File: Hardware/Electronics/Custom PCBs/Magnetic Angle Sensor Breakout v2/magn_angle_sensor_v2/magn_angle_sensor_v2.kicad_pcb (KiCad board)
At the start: 2 copper layers, 25 x 25 mm, 57 parts, among them J1 JST PH 01x04, J2 USB C Receptacle, J3 120TR, SW1 USB_BOOT, SW2 RESET, U1 MT6701-CT, U2 RP2040, U3 W25Q128JVS, U4 SE8650X2-HF, U5 SN65HVD1050D, U6 XC6206P332MR, Y1 12MHz/12pF/50Ω/20ppm

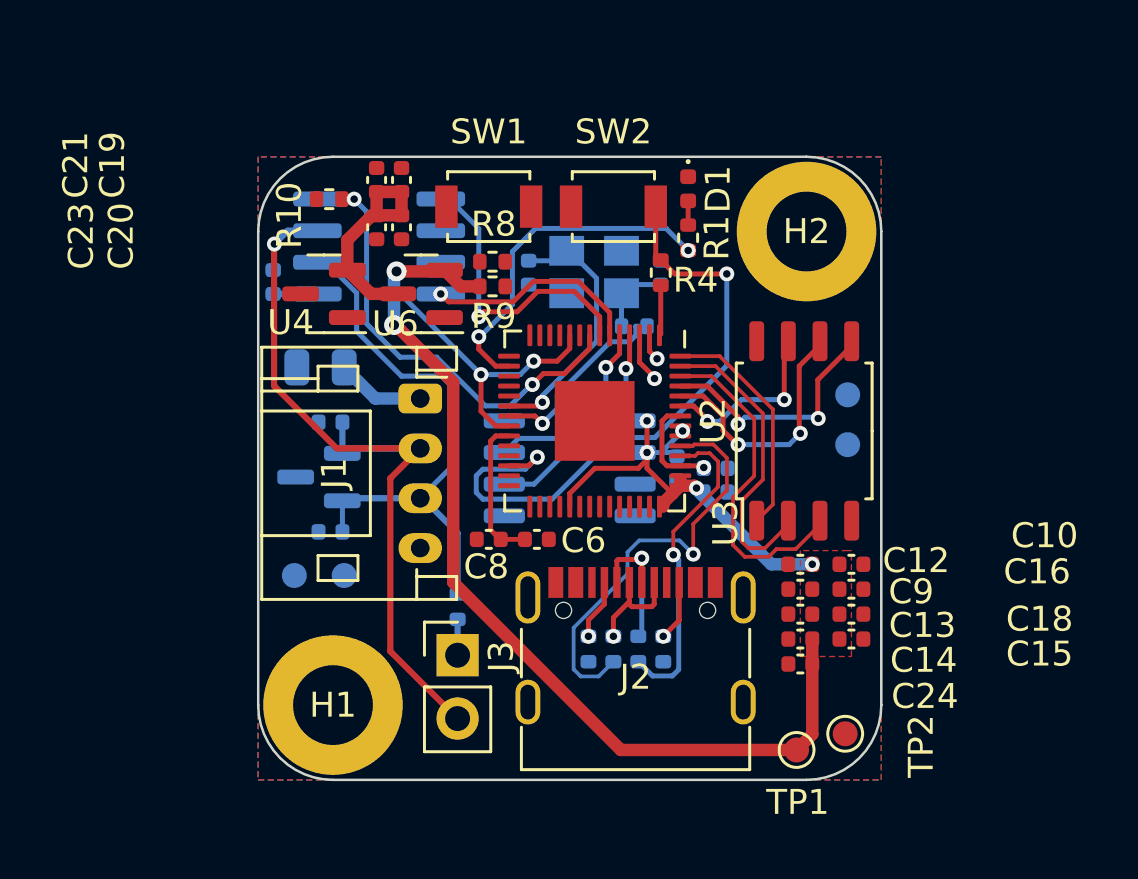
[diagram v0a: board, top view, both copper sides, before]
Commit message: Finish CAN Magnetic Angle Sensor v2
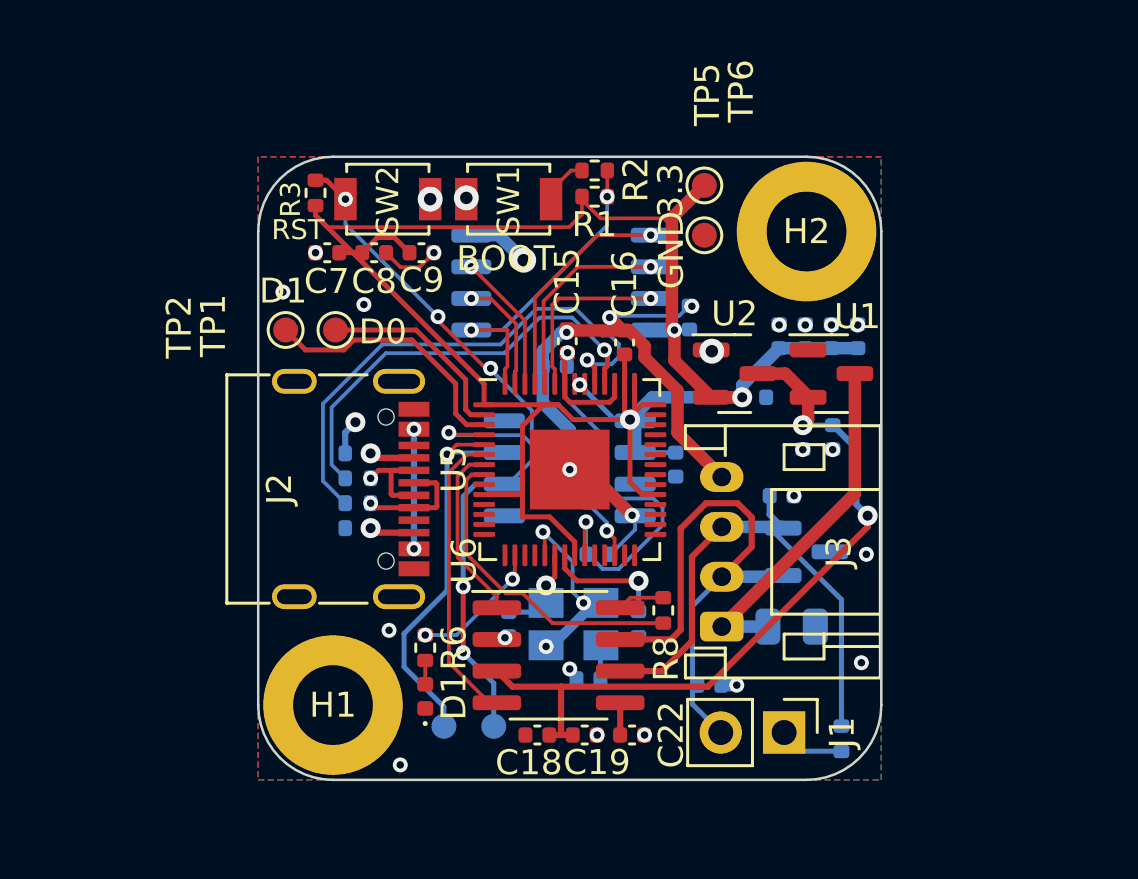
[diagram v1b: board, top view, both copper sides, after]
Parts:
- C10: value 100n -> 1u/100V; footprint Capacitor_SMD:C_0402_1005Metric -> Capacitor_SMD:C_0805_2012Metric; moved to B.Cu
- C12, C13: value 100n -> 1u; moved to B.Cu
- C14, C6, U3: moved to B.Cu
- C15, C16, C18: value 100n -> 1u
- C17: value 1u/100V -> 100n; footprint Capacitor_SMD:C_0805_2012Metric -> Capacitor_SMD:C_0402_1005Metric
- C19: value 1u -> 100n
- C2, C3: value 47p -> 100n
- C20: value 1u -> 22p; moved to B.Cu
- C21: value 100n -> 22p; moved to B.Cu
- C22: moved to F.Cu
- C23, C24: value 1u -> 47p; moved to B.Cu
- C4, C5: value 22p -> 100n
- C7: value 1u -> 100n; moved to F.Cu
- J1: value JST PH 01x04 -> 120TR; footprint Connector_JST:JST_PH_S4B-PH-K_1x04_P2.00mm_Horizontal -> Connector_PinHeader_2.54mm:PinHeader_1x02_P2.54mm_Vertical
- J3: value 120TR -> JST PH 01x04; footprint Connector_PinHeader_2.54mm:PinHeader_1x02_P2.54mm_Vertical -> Connector_JST:JST_PH_S4B-PH-K_1x04_P2.00mm_Horizontal
- R1: value 10k -> 10K
- R10: value NC -> 5.1k; moved to B.Cu
- R11: value 120 -> 5.1k
- R2: value 5.1k -> 1K; moved to F.Cu
- R3: value 5.1k -> 10k; moved to F.Cu
- R4: value 10k -> 27.4; moved to B.Cu
- R6: value 27.4 -> 10k; moved to F.Cu
- R8: value 1K -> NC
- R9: value 10K -> 120; moved to B.Cu
- SW1: value USB_BOOT -> BOOT
- TP1: value 3.3V -> D0
- TP2: value GND -> D1
- TP5: value D0 -> 3.3V; moved to F.Cu
- TP6: value D1 -> GND; moved to F.Cu
- U1: value MT6701-CT -> SE8650X2-HF; footprint Package_SO:SOP-8_3.9x4.9mm_P1.27mm -> Package_TO_SOT_SMD:SOT-23; moved to F.Cu
- U2: value RP2040 -> XC6206P332MR; footprint Package_DFN_QFN:QFN-56-1EP_7x7mm_P0.4mm_EP3.2x3.2mm -> Package_TO_SOT_SMD:SOT-23
- U4: value SE8650X2-HF -> MT6701-CT; footprint Package_TO_SOT_SMD:SOT-23 -> Package_SO:SOP-8_3.9x4.9mm_P1.27mm; moved to B.Cu
- U5: value SN65HVD1050D -> RP2040; footprint Package_SO:SOIC-8_3.9x4.9mm_P1.27mm -> Package_DFN_QFN:QFN-56-1EP_7x7mm_P0.4mm_EP3.2x3.2mm; moved to F.Cu
- U6: value XC6206P332MR -> SN65HVD1050D; footprint Package_TO_SOT_SMD:SOT-23 -> Package_SO:SOIC-8_3.9x4.9mm_P1.27mm
- moved TP2 27.7 mm to (21.1, 26.9)
- moved TP1 25.0 mm to (23.1, 26.9)
- moved C19 23.8 mm to (33.1, 43.2), turned to 180 degrees
- moved C22 23.2 mm to (35.0, 43.2), turned to 0 degrees
- moved D1 22.9 mm to (26.7, 41.6), turned to 90 degrees
- moved R9 22.9 mm to (43.4, 43.4), turned to 90 degrees
- moved C3 22.6 mm to (44.0, 27.2), turned to -90 degrees
- moved C23 22.1 mm to (38.1, 41.2), turned to 0 degrees
- moved C21 21.4 mm to (33.2, 41.0), turned to 0 degrees
- moved R3 21.3 mm to (22.3, 21.4), turned to 90 degrees
- moved C9 21.3 mm to (26.6, 23.9)
- moved J1 19.8 mm to (41.1, 43.1)
- moved CR1 19.8 mm to (42.0, 35.9), turned to 0 degrees
- moved R2 19.4 mm to (33.5, 20.6), turned to 0 degrees
- moved C7 17.8 mm to (22.8, 23.9), turned to 0 degrees
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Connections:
- C1 pad 1: +3.3V -> GND
- C1 pad 2: GND -> +1V1
- C10 pad 1: +3.3V -> GND
- C10 pad 2: GND -> +24V
- C11 pad 1: +3.3V -> +5V
- C12 pad 1: GND -> +5V
- C12 pad 2: +3.3V -> GND
- C13 pad 1: GND -> +3.3V
- C13 pad 2: +3.3V -> GND
- C14 pad 1: GND -> +3.3V
- C14 pad 2: +3.3V -> GND
- C15 pad 2: +3.3V -> +1V1
- C16 pad 1: GND -> +3.3V
- C16 pad 2: +3.3V -> GND
- C17 pad 1: GND -> +3.3V
- C17 pad 2: +24V -> GND
- C18 pad 2: +3.3V -> +5V
- C2 pad 1: /CAN_H -> GND
- C2 pad 2: GND -> +1V1
- C20 pad 1: +5V -> GND
- C20 pad 2: GND -> Net-(U5-XIN)
- C21 pad 2: +5V -> Net-(C21-Pad2)
- C22 pad 1: Net-(U5-VREF) -> Net-(U6-VREF)
- C23 pad 1: +5V -> /CAN_H
- C24 pad 1: +3.3V -> /CAN_L
- C3 pad 1: /CAN_L -> GND
- C3 pad 2: GND -> +3.3V
- C4 pad 2: Net-(U2-XIN) -> +3.3V
- C5 pad 2: Net-(C5-Pad2) -> +3.3V
- C6 pad 2: +1V1 -> +3.3V
- C7 pad 2: +1V1 -> +3.3V
- C8 pad 2: +1V1 -> +3.3V
- J1 pad 1: +24V -> Net-(J1-Pin_1)
- J3 pad 1: Net-(J3-Pin_1) -> +24V
- R1 pad 1: Net-(D1-A) -> /QSPI_SS
- R1 pad 2: /LED -> +3.3V
- R10 pad 1: Net-(U5-S) -> Net-(J2-CC2)
- R10 pad 2: /CAN_S -> GND
- R11 pad 1: Net-(J3-Pin_1) -> Net-(J2-CC1)
- R11 pad 2: /CAN_L -> GND
- R2 pad 1: Net-(J2-CC2) -> /~{USB_BOOT}
- R2 pad 2: GND -> /QSPI_SS
- R3 pad 1: Net-(J2-CC1) -> +3.3V
- R3 pad 2: GND -> /RUN
- R4 pad 1: +3.3V -> /USB_D+
- R4 pad 2: /RUN -> Net-(U5-USB_DP)
- R5 pad 1: /USB_D+ -> Net-(U5-USB_DM)
- R5 pad 2: Net-(U2-USB_DP) -> /USB_D-
- R6 pad 1: Net-(U2-USB_DM) -> Net-(D1-A)
- R6 pad 2: /USB_D- -> /LED
- R7 pad 1: Net-(C5-Pad2) -> Net-(C21-Pad2)
- R7 pad 2: Net-(U2-XOUT) -> Net-(U5-XOUT)
- R8 pad 1: /~{USB_BOOT} -> Net-(U6-S)
- R8 pad 2: /QSPI_SS -> /CAN_S
- R9 pad 1: /QSPI_SS -> Net-(J1-Pin_1)
- R9 pad 2: +3.3V -> /CAN_L
- TP1 pad 1: +3.3V -> Net-(U5-GPIO0)
- TP2 pad 1: GND -> Net-(U5-GPIO1)
- TP5 pad 1: Net-(U2-GPIO0) -> +3.3V
- TP6 pad 1: Net-(U2-GPIO1) -> GND
- U1 pad 1: +3.3V -> GND
- U1 pad 2: +3.3V -> +5V
- U1 pad 3: unconnected-(U1-ANALOG/PWM-Pad3) -> +24V
- U2 pad 1: +3.3V -> GND
- U2 pad 2: Net-(U2-GPIO0) -> +3.3V
- U2 pad 3: Net-(U2-GPIO1) -> +5V
- U4 pad 1: GND -> +3.3V
- U4 pad 2: +5V -> +3.3V
- U4 pad 3: +24V -> unconnected-(U4-ANALOG/PWM-Pad3)
- U5 pad 1: /CAN_TX -> +3.3V
- U5 pad 2: GND -> Net-(U5-GPIO0)
- U5 pad 3: +5V -> Net-(U5-GPIO1)
- U5 pad 4: /CAN_RX -> /SDA
- U5 pad 5: Net-(U5-VREF) -> /SCL
- U5 pad 6: /CAN_L -> /CAN_RX
- U5 pad 7: /CAN_H -> /CAN_TX
- U5 pad 8: Net-(U5-S) -> /CAN_S
- U6 pad 1: GND -> /CAN_TX
- U6 pad 2: +3.3V -> GND
- Y1 pad 1: Net-(C5-Pad2) -> Net-(C21-Pad2)
- Y1 pad 3: Net-(U2-XIN) -> Net-(U5-XIN)
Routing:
- net GND: track 0.00 -> 40.2 mm, vias 0 -> 33
- net Net-(U5-USB_DP): track 0.00 -> 21.5 mm, vias 0 -> 1
- net +5V: track 9.09 -> 30.2 mm, vias 0 -> 2
- net Net-(U5-USB_DM): track 0.00 -> 17.5 mm, vias 0 -> 1
- net Net-(U2-USB_DP): track 17.1 -> 0.00 mm, vias 1 -> 0
- net +3.3V: track 72.5 -> 88.0 mm, vias 9 -> 4
- net Net-(U2-USB_DM): track 12.8 -> 0.00 mm, vias 1 -> 0
- net +1V1: track 10.1 -> 22.0 mm, vias 1 -> 2
- net +24V: track 3.57 -> 14.2 mm
- net Net-(U2-XIN): track 10.6 -> 0.00 mm, vias 1 -> 0
- net Net-(U5-GPIO1): track 0.00 -> 10.6 mm
- net /SDA: track 8.75 -> 18.7 mm, vias 1 -> 3
- net /CAN_H: track 31.5 -> 22.7 mm, vias 1 -> 0
- net /SCL: track 7.73 -> 16.3 mm
- net /LED: track 13.8 -> 5.43 mm
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- removed copper zone on F.Cu, net +3.3V
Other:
- board text added: "3.3"
- board text added: "BOOT"
- board text added: "D0"
- board text added: "D1"
- board text added: "GND"
- board text added: "RST"
- board text added: "SDASDL"
